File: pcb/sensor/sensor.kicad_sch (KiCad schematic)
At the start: 40 parts, among them J3 sig_in, J4 sig_out, J5 Conn_01x02_Pin, J6 Conn_01x02_Pin, J7 Conn_02x02_Counter_Clockwise, U1 TJA1051T-3, U2 HX711, U5 LMR16030SDDAR, U6 LM2596S-3.3, U7 LM2596S-5

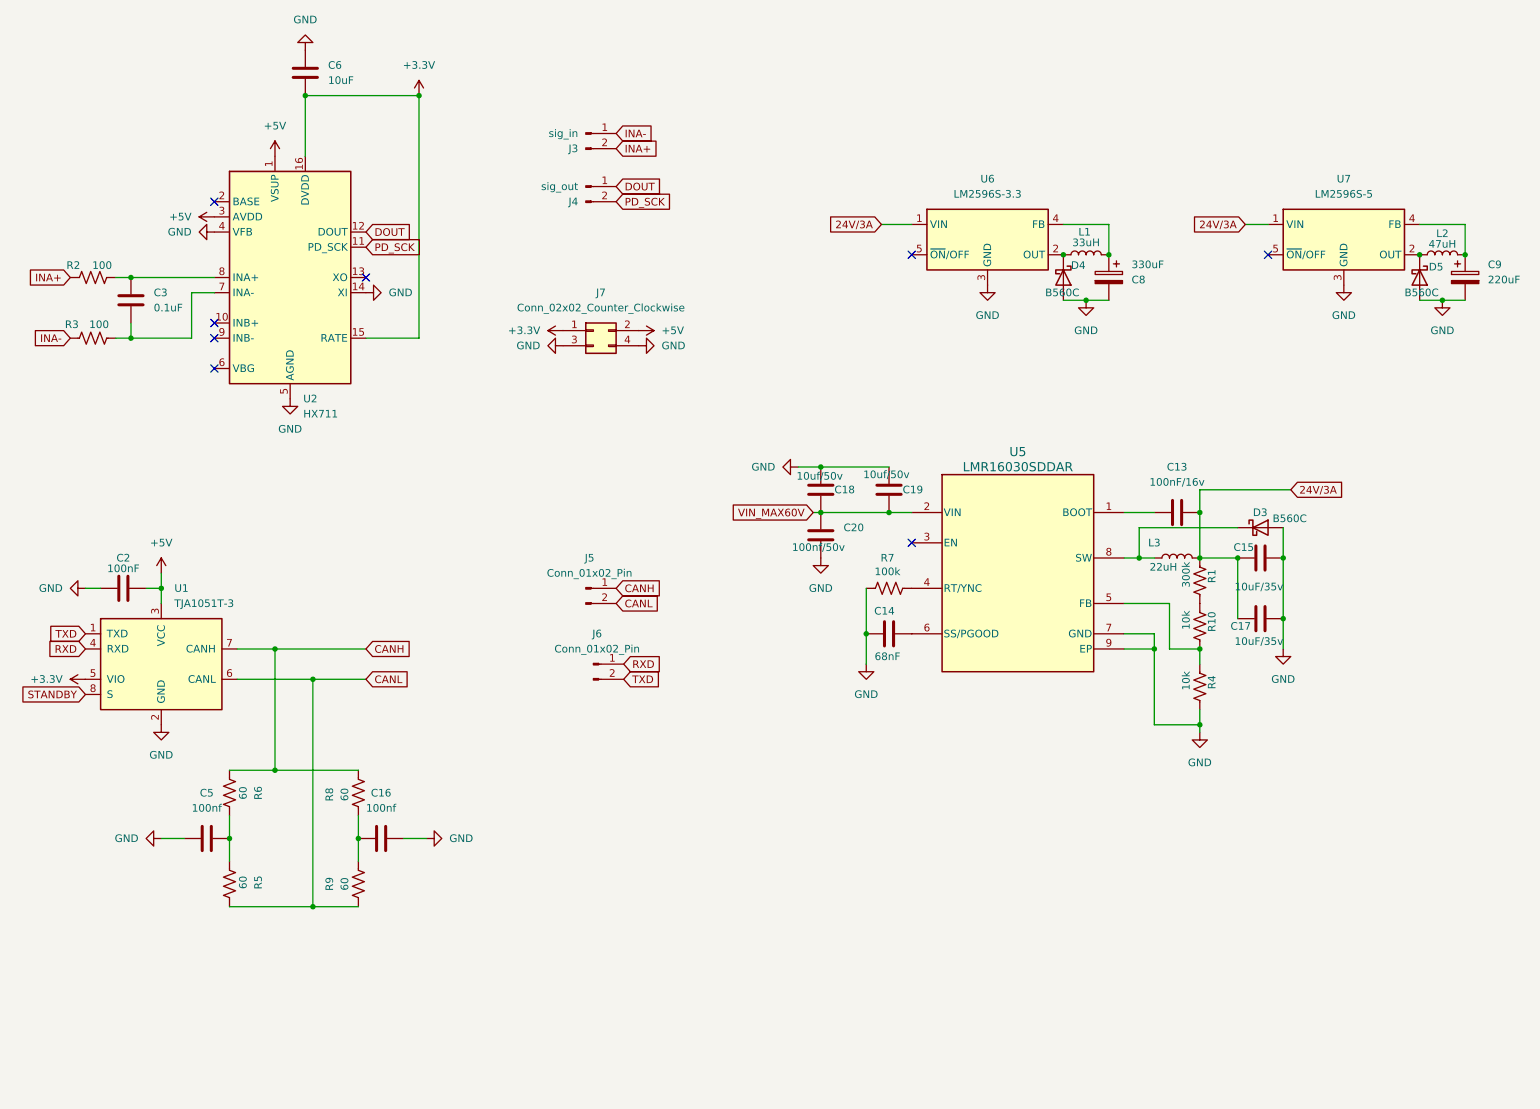
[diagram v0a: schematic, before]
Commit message: feat: add dc-dc compute script
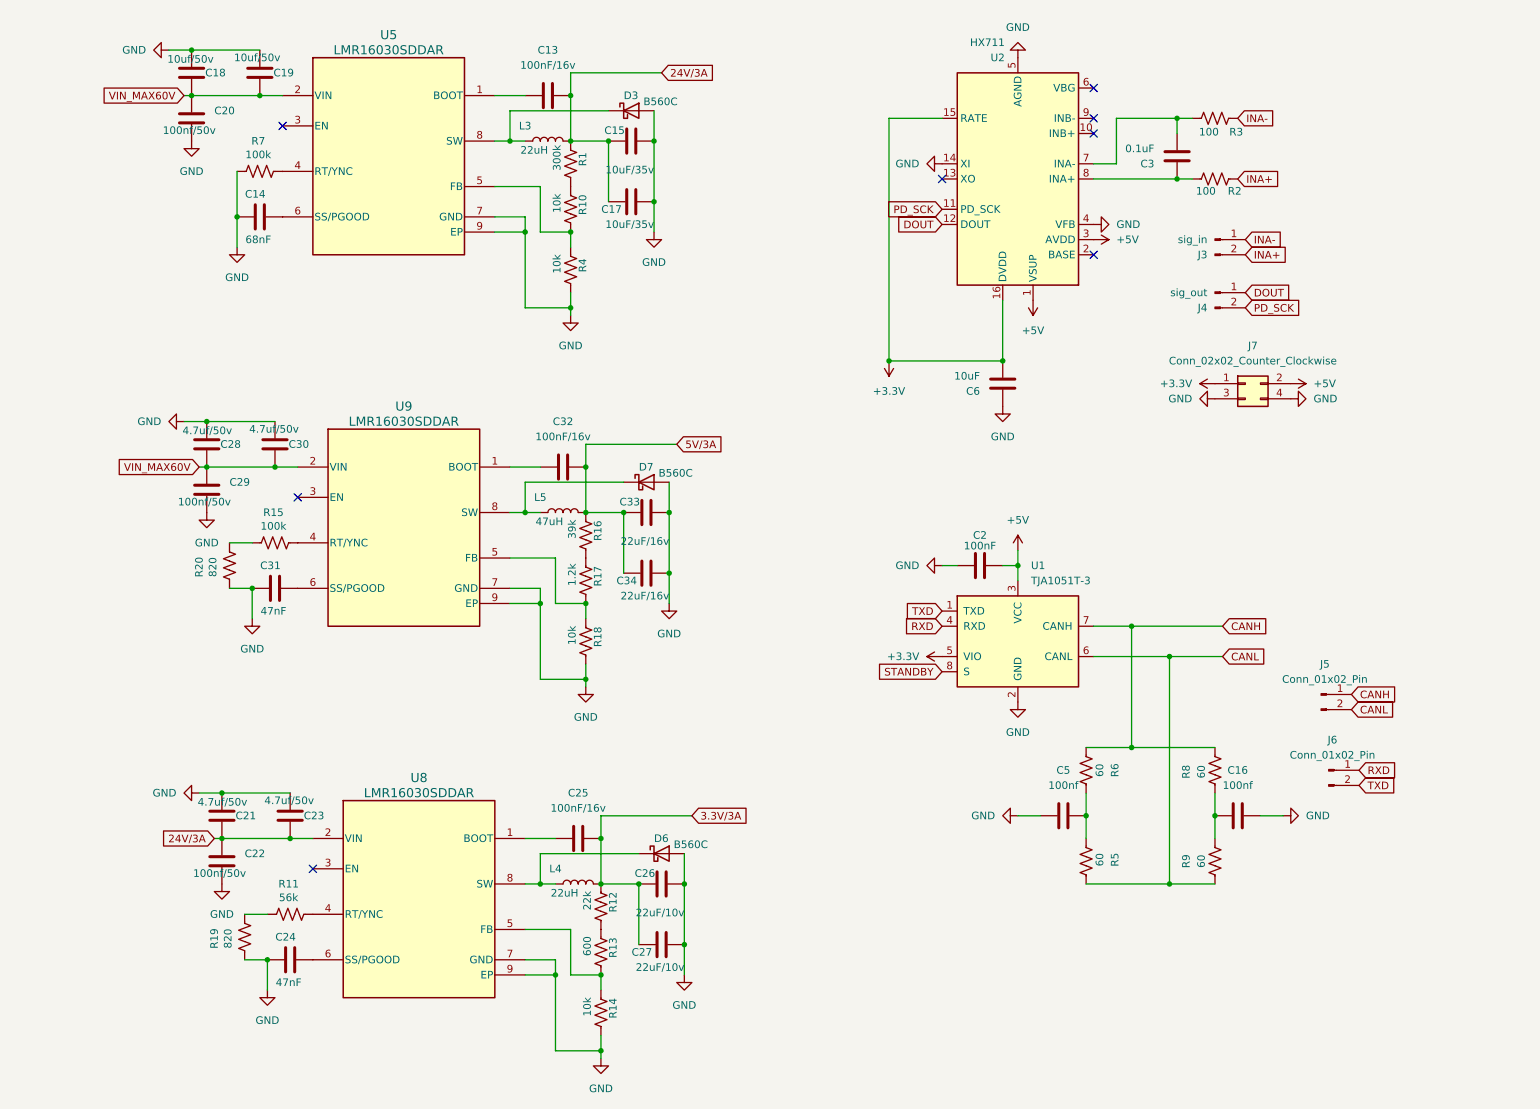
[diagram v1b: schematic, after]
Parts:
- removed C8: 330uF, symbol Device:C_Polarized
- removed C9: 220uF, symbol Device:C_Polarized
- removed D4, D5: B560C, Diode_SMD:D_SMC, symbol Device:D_Schottky
- removed L1: 33uH, symbol Device:L
- removed L2: 47uH, symbol Device:L
- removed U6: LM2596S-3.3, Package_TO_SOT_SMD:TO-263-5_TabPin3, symbol Regulator_Switching:LM2596S-3.3
- removed U7: LM2596S-5, Package_TO_SOT_SMD:TO-263-5_TabPin3, symbol Regulator_Switching:LM2596S-5
- added C21, C23, C28, C30: 4.7uf/50v, Capacitor_SMD:C_1210_3225Metric, symbol Device:C
- added C22, C29: 100nf/50v, Capacitor_SMD:C_1210_3225Metric, symbol Device:C
- added C24, C31: 47nF, Capacitor_SMD:C_0603_1608Metric, symbol Device:C
- added C25, C32: 100nF/16v, Capacitor_SMD:C_0603_1608Metric, symbol Device:C
- added C26: 22uF/10v, Capacitor_SMD:C_1206_3216Metric, symbol Device:C
- added C27: 22uF/10v, Capacitor_SMD:C_1210_3225Metric, symbol Device:C
- added C33: 22uF/16v, Capacitor_SMD:C_1206_3216Metric, symbol Device:C
- added C34: 22uF/16v, Capacitor_SMD:C_1210_3225Metric, symbol Device:C
- added D6, D7: B560C, Diode_SMD:D_SMC, symbol Device:D_Schottky
- added L4: 22uH, Inductor_SMD:L_Changjiang_FXL0650, symbol Device:L
- added L5: 47uH, Inductor_SMD:L_Changjiang_FXL0650, symbol Device:L
- added R11: 56k, Resistor_SMD:R_0603_1608Metric, symbol Device:R_US
- added R12: 22k, Resistor_SMD:R_0603_1608Metric, symbol Device:R_US
- added R13: 600, Resistor_SMD:R_0603_1608Metric, symbol Device:R_US
- added R14, R18: 10k, Resistor_SMD:R_0603_1608Metric, symbol Device:R_US
- added R15: 100k, Resistor_SMD:R_0603_1608Metric, symbol Device:R_US
- added R16: 39k, Resistor_SMD:R_0603_1608Metric, symbol Device:R_US
- added R17: 1.2k, Resistor_SMD:R_0603_1608Metric, symbol Device:R_US
- added R19, R20: 820, Resistor_SMD:R_0603_1608Metric, symbol Device:R_US
- added U8, U9: LMR16030SDDAR, Package_SO:TI_SO-PowerPAD-8_ThermalVias, symbol 2025-01-08_11-11-09:LMR16030SDDAR
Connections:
- net 24V/3A: now also C21.1, C22.1, C23.2, U8.2 (VIN)
- net GND: now also C21.2, C22.2, C23.1, C24.2, C26.2, C27.1, C28.2, C29.2, C30.1, C31.2, C33.2, C34.1, D6.2 (A), D7.2 (A), R14.2, R18.2, R19.2, R20.2, U8.7 (GND), U8.9 (EP), U9.7 (GND), U9.9 (EP)
- net VIN_MAX60V: now also C28.1, C29.1, C30.2, U9.2 (VIN)
- new net: C25.2, U8.1 (BOOT)
- new net: D6.1 (K), L4.1, U8.8 (SW)
- new net: R16.2, R17.1
- new net: R17.2, R18.1, U9.5 (FB)
- new net: R15.2, R20.1
- new net: R13.2, R14.1, U8.5 (FB)
- new net: D7.1 (K), L5.1, U9.8 (SW)
- new net: C31.1, U9.6 (SS/PGOOD)
- new net: C32.2, U9.1 (BOOT)
- new net: R15.1, U9.4 (RT/YNC)
- new net: R12.2, R13.1
- new net: R11.1, U8.4 (RT/YNC)
- new net: R11.2, R19.1
- new net: C24.1, U8.6 (SS/PGOOD)
- new net 3.3V/3A: C25.1, C26.1, C27.2, L4.2, R12.1
- new net 5V/3A: C32.1, C33.1, C34.2, L5.2, R16.1
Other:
- moved on the sheet: C13, C14, C15, C16, C17, C18, C19, C2, C20, C3, C5, C6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
